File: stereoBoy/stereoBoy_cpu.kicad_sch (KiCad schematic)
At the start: 42 parts, among them J2 JST_1mm_3_Vertical, J3 GameBoy_Cartridge, J4 Conn_01x02, J8 Conn_01x02, SW1 SMD_4.6x2.8mm_h2.5mm, SW2 SMD_4.6x2.8mm_h2.5mm, U11 RP2350B, U14 DS3231MZ, Y3 32.768kHz

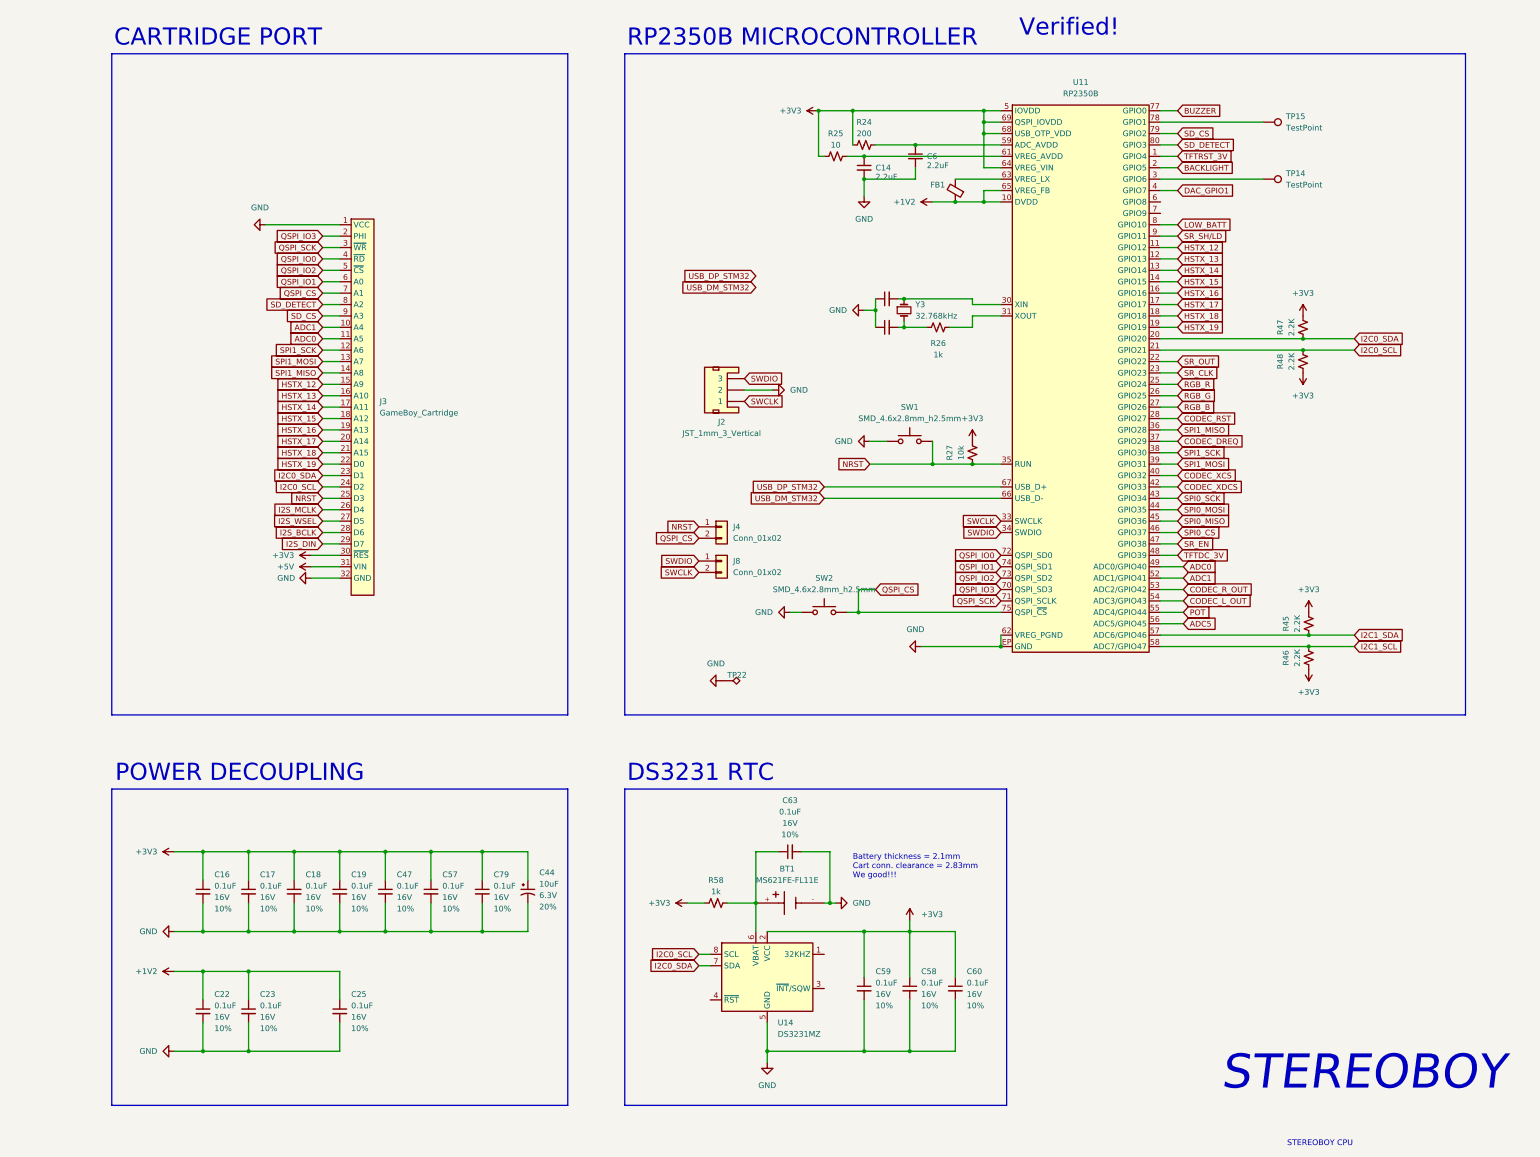
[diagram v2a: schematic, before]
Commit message: yuh
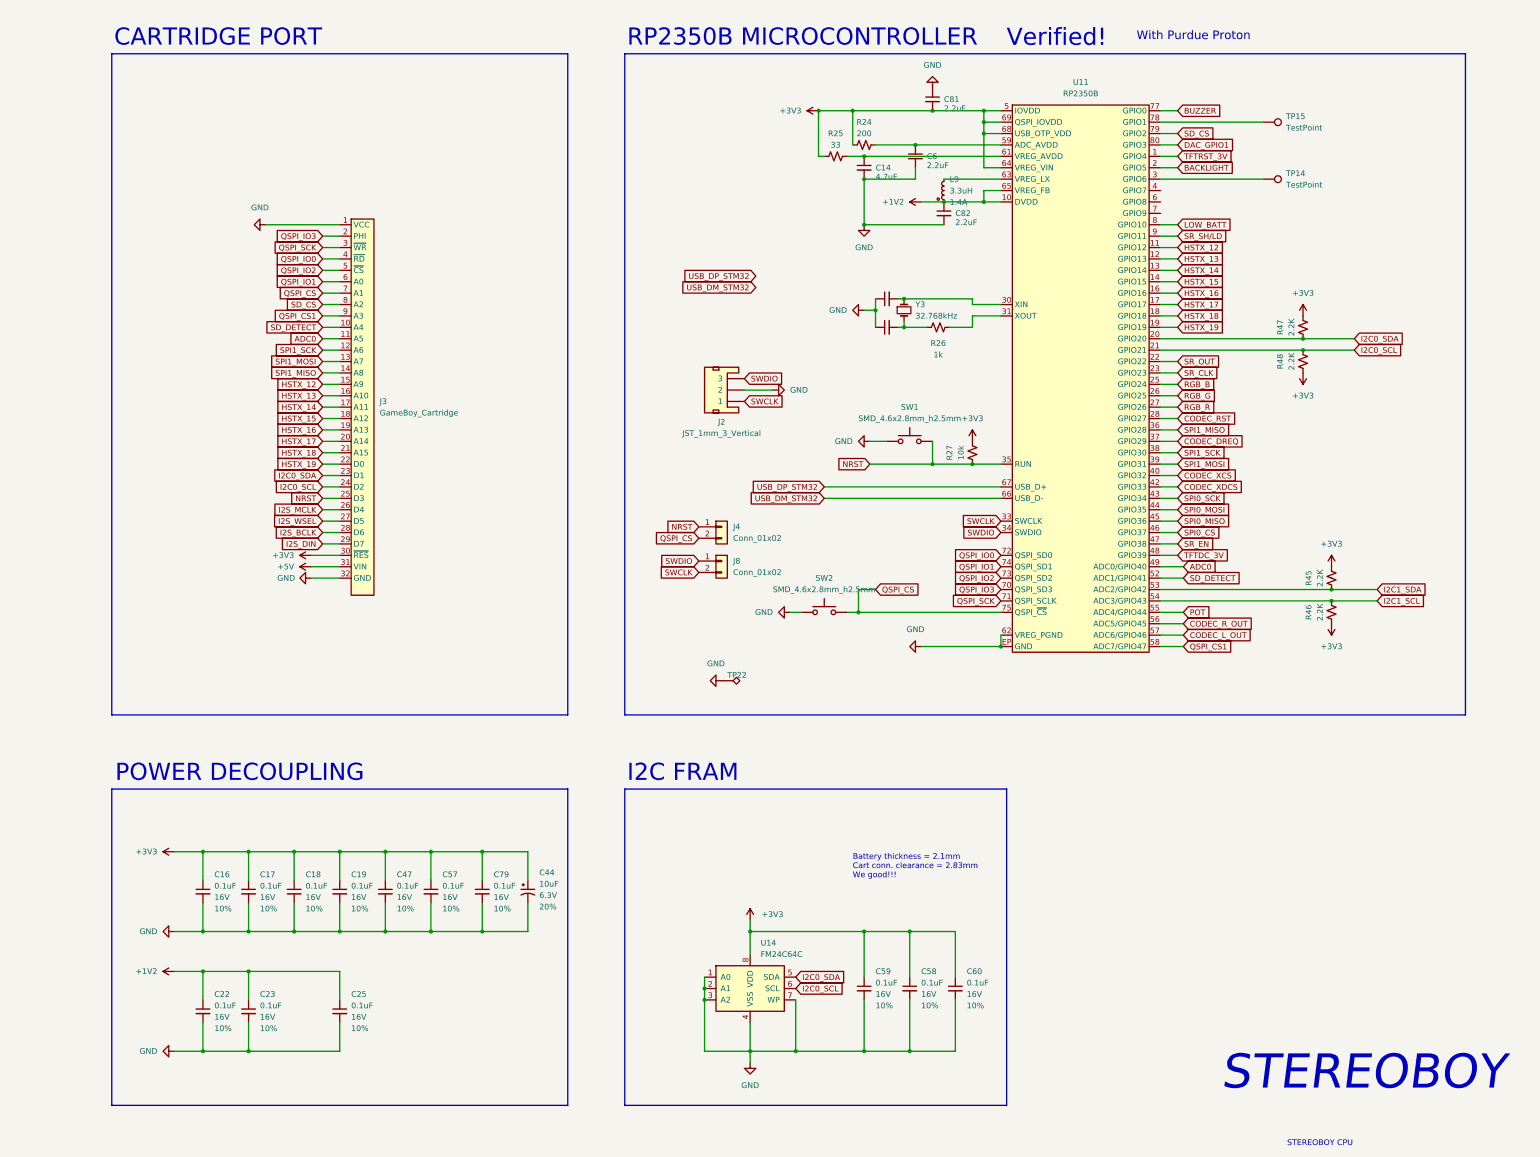
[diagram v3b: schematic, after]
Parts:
- removed BT1: MS621FE-FL11E, MS621FE_FL11E:MS621FE_FL11E, symbol MS621FE-FL11E:MS621FE-FL11E
- removed C63: 0.1uF, SparkFun-Capacitor:C_0402_1005Metric, symbol SparkFun-Capacitor:0.1uF_0402_16V_10%
- removed FB1: FerriteBead_Small, Inductor_SMD:L_0402_1005Metric, symbol Device:FerriteBead_Small
- removed R58: 1k, Resistor_SMD:R_0402_1005Metric, symbol SparkFun-Resistor:330_0603
- removed U14: DS3231MZ, Package_SO:SOIC-8_3.9x4.9mm_P1.27mm, symbol Timer_RTC:DS3231MZ
- added C81, C82: 2.2uF, Worthington_Assembly:WAi_0402_1005Metric, symbol Device:C_Small
- added L9: 3.3uH, Inductor_SMD:L_Cenker_CKCS201610, symbol SparkFun-Coil:3.3uH_0806_1.4A_Polarized
- added U14: FM24C64C, Package_SO:SOIC-8_3.9x4.9mm_P1.27mm, symbol Memory_NVRAM:FM24C64C
- C14: value 2.2uF -> 4.7uF
- R25: value 10 -> 33
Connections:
- net ADC1 is gone; now on net SD_DETECT: J3.10 (A4), U11.52 (ADC1/GPIO41)
- net ADC5 is gone; now on net CODEC_R_OUT: U11.56 (ADC5/GPIO45)
- net +1V2: now also C82.1, L9.1
- net +3V3: now also C81.2, U14.8 (VDD)
- net CODEC_L_OUT: now also U11.57 (ADC6/GPIO46); no longer U11.54 (ADC3/GPIO43)
- net CODEC_R_OUT: no longer U11.53 (ADC2/GPIO42)
- net DAC_GPIO1: now also U11.80 (GPIO3); no longer U11.4 (GPIO7)
- net GND: now also C81.1, C82.2, U14.1 (A0), U14.2 (A1), U14.3 (A2), U14.4 (VSS), U14.7 (WP)
- net I2C0_SCL: now also U14.6 (SCL)
- net I2C0_SDA: now also U14.5 (SDA)
- net I2C1_SCL: now also U11.54 (ADC3/GPIO43); no longer U11.58 (ADC7/GPIO47)
- net I2C1_SDA: now also U11.53 (ADC2/GPIO42); no longer U11.57 (ADC6/GPIO46)
- net RGB_B: now also U11.25 (GPIO24); no longer U11.27 (GPIO26)
- net RGB_R: now also U11.27 (GPIO26); no longer U11.25 (GPIO24)
- net SD_CS: now also J3.8 (A2); no longer J3.9 (A3)
- net SD_DETECT: no longer J3.8 (A2), U11.80 (GPIO3)
- net at U11.63 (VREG_LX): now also L9.2
- new net QSPI_CS1: J3.9 (A3), U11.58 (ADC7/GPIO47)
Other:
- note added: "I2C FRAM"
- note added: "With Purdue Proton"
- note removed: "DS3231 RTC"
- moved on the sheet: R45, R46
